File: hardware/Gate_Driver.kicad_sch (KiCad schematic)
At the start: 30 parts, among them U1 DRV8323RSRGZR

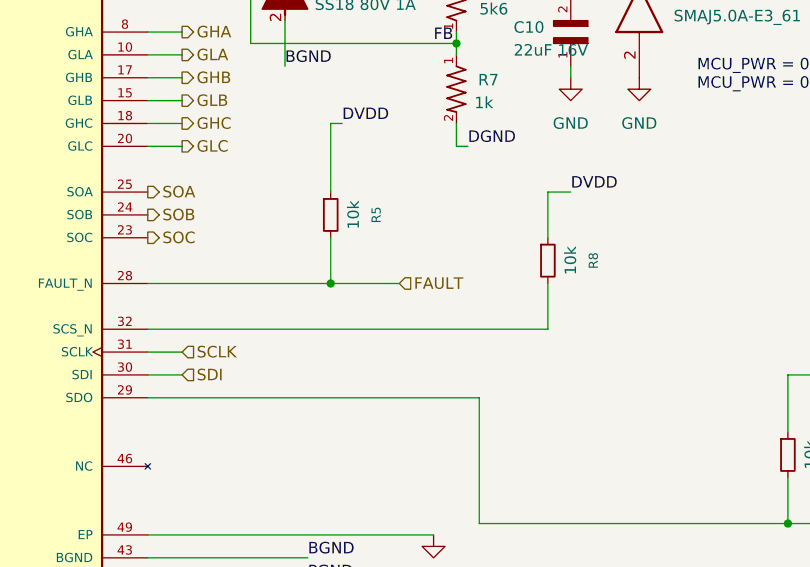
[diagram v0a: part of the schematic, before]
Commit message: final project board layout is in this commit
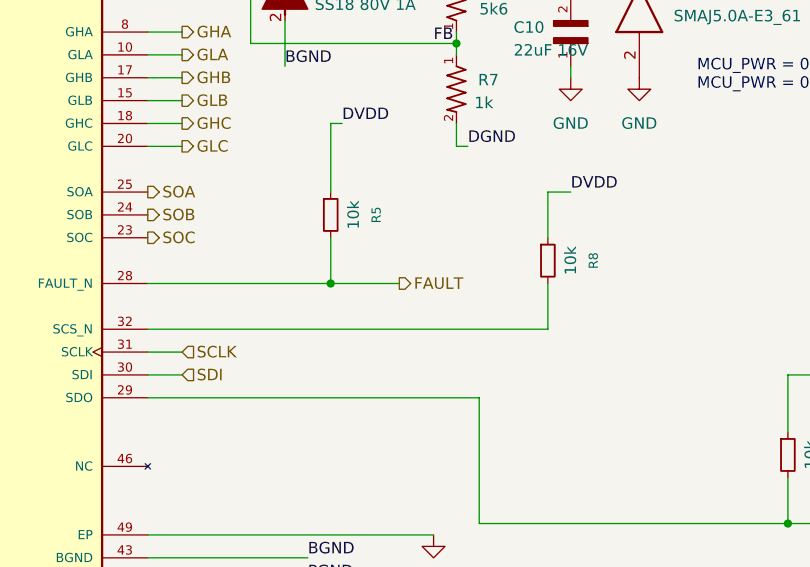
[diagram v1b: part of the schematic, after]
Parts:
- C11: footprint 08056D104KAT2A:CAPC2012X140N -> Capacitor_SMD:C_0805_2012Metric_Pad1.18x1.45mm_HandSolder
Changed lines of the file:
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@@
 	)
 	(hierarchical_label "FAULT"
-		(shape input)
+		(shape output)
 		(at 125.73 97.79 0)
 		(effects
@@
 			)
 		)
-		(property "Footprint" "08056D104KAT2A:CAPC2012X140N"
+		(property "Footprint" "Capacitor_SMD:C_0805_2012Metric_Pad1.18x1.45mm_HandSolder"
 			(at 157.48 46.99 0)
 			(effects
